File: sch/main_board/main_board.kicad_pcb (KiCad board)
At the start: 2 copper layers, 94.8 x 75.2 mm, 58 parts, among them J1 BVCC, J13 5V_GND, J14 IO23, J15 IO22, J16 IO1, J17 IO3, J18 IO21, J2 BGND, J21 5V, J22 TX2, J23 RX2, J24 12V_CUT2, J25 12V_CUT, J26 DC 12V, J27 DC 5V, J3 3.3V, J30 5V_CUT, J4 PWR_MOTOR_L, J5 PWR_MOTOR_R, J6 CUT_LOAD, J7 MOTOR_R, J8 MOTOR_L, J9 EN, Q1 BC847, Q2 K4145, Q3 K4145, Q4 BC847, Q5 K4145, Q6 BC847, Q7 K4145, Q8 BC847, Q9 K4145

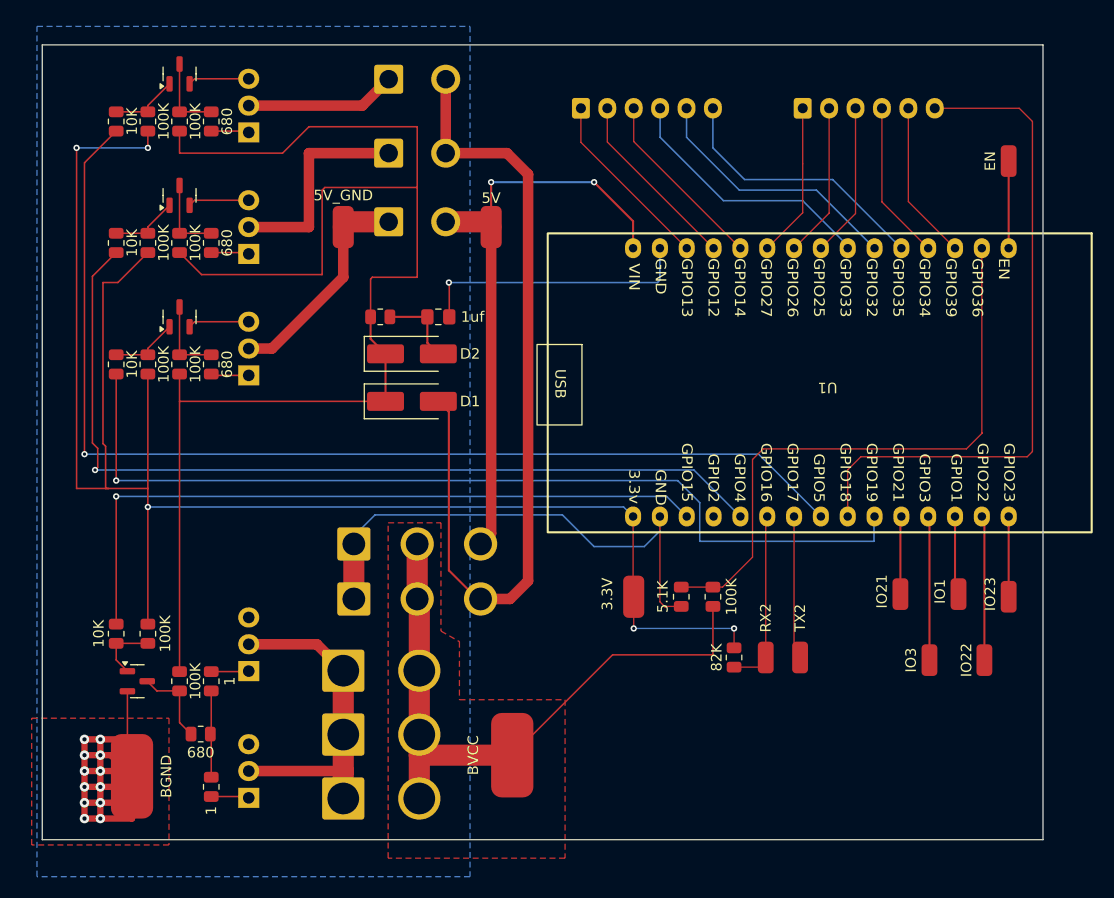
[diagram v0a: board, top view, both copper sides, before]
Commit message: Final scheme changes before production
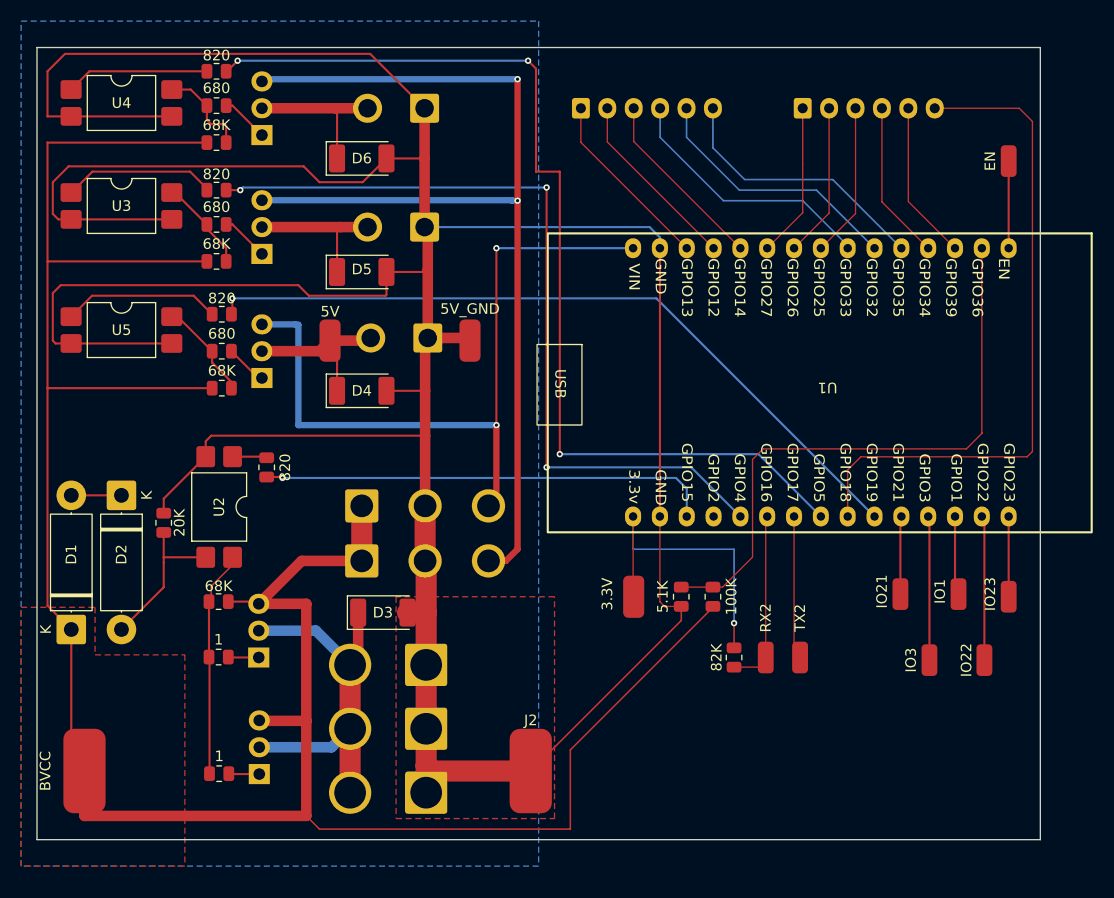
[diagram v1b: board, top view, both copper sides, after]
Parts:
- removed C1: 1uf, Capacitor_SMD:C_0805_2012Metric_Pad1.18x1.45mm_HandSolder
- removed Q6, Q8: BC847, Package_TO_SOT_SMD:SOT-23
- removed Q7, Q9: K4145, Package_TO_SOT_THT:TO-220-3_Vertical
- removed R15: 10K, Resistor_SMD:R_0805_2012Metric
- removed R16, R17: 100K, Resistor_SMD:R_0805_2012Metric
- removed R18: 680, Resistor_SMD:R_0805_2012Metric
- removed R21: 100, Resistor_SMD:R_0805_2012Metric
- added D3: D, Diode_SMD:D_2010_5025Metric_Pad1.52x2.65mm_HandSolder, F.Cu at (88.8, 93.5)
- added D4: D, Diode_SMD:D_2010_5025Metric_Pad1.52x2.65mm_HandSolder, F.Cu at (86.8, 72.5)
- added D5: D, Diode_SMD:D_2010_5025Metric_Pad1.52x2.65mm_HandSolder, F.Cu at (86.8, 61.2)
- added D6: D, Diode_SMD:D_2010_5025Metric_Pad1.52x2.65mm_HandSolder, F.Cu at (86.8, 50.5)
- added U2: EL817, Package_DIP:SMDIP-4_W9.53mm, F.Cu at (73.2, 83.5)
- added U3: EL817, Package_DIP:SMDIP-4_W9.53mm, F.Cu at (64.0, 55.0)
- added U4: EL817, Package_DIP:SMDIP-4_W9.53mm, F.Cu at (64.0, 45.2)
- added U5: EL817, Package_DIP:SMDIP-4_W9.53mm, F.Cu at (64.0, 66.8)
- D1, D2: value D -> 5.1; footprint Diode_SMD:D_SMA_Handsoldering -> Diode_THT:D_5W_P12.70mm_Horizontal
- Q1, Q4: value BC847 -> IRF4905; footprint Package_TO_SOT_SMD:SOT-23 -> Package_TO_SOT_THT:TO-220-3_Vertical; moved to B.Cu
- Q2, Q3, Q5: value K4145 -> IRF4905
- R1: value 10K -> 20K
- R10: value 680 -> 1
- R11: value 10K -> 1
- R12, R13: value 100K -> 680
- R2, R9: value 100K -> 68K
- R3, R8: value 100K -> 820
- R4: value 680 -> 820
- R5: value 1 -> 68K
- R6: value 1 -> 820
- R7: value 10K -> 68K
- moved R6 67.8 mm to (73.0, 42.2), turned to 0 degrees
- moved Q3 62.8 mm to (77.3, 48.3)
- moved R4 51.5 mm to (73.0, 53.5)
- moved R11 51.2 mm to (73.2, 108.8), turned to 180 degrees
- moved J1 40.5 mm to (60.5, 108.5)
- moved R5 39.8 mm to (73.0, 60.2), turned to 180 degrees
- moved Q2 39.5 mm to (77.3, 59.5)
- moved D1 38.8 mm to (59.2, 95.1), turned to 90 degrees
- moved Q5 37.8 mm to (77.0, 108.8)
- moved J2 37.8 mm to (102.8, 108.5)
- moved D2 30.6 mm to (64.0, 82.4), turned to -90 degrees
- moved R10 27.7 mm to (73.2, 97.7), turned to 180 degrees
- moved R7 23.0 mm to (73.0, 49.0), turned to 180 degrees
- moved R3 21.9 mm to (77.8, 79.8), turned to -90 degrees
- moved J21 18.7 mm to (83.8, 67.8)
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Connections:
- D1 pad 1: MF_VCC -> VCC
- D1 pad 2: +12V -> Net-(D1-A)
- D2 pad 1: MF_VCC -> Net-(D1-A)
- D2 pad 2: Net-(D2-A) -> MF_GND
- J13 pad 1: Net-(J13-Pin_1) -> GND
- J21 pad 1: +5V -> Net-(D4-K)
- J24 pad 1: Net-(J24-Pin_1) -> GND
- J24 pad 2: +12V -> Net-(D6-K)
- J25 pad 1: Net-(J25-Pin_1) -> GND
- J25 pad 2: +12V -> Net-(D5-K)
- J26 pad 1: GND -> VCC
- J26 pad 2: VCC -> GND
- J27 pad 1: GND -> VCC
- J27 pad 2: VCC -> GND
- J30 pad 1: Net-(J13-Pin_1) -> GND
- J30 pad 2: +5V -> Net-(D4-K)
- J4 pad 1: Net-(J4-Pin_1) -> GND
- J4 pad 2: VCC -> Net-(D3-K)
- J5 pad 1: Net-(J4-Pin_1) -> GND
- J5 pad 2: VCC -> Net-(D3-K)
- J6 pad 1: Net-(J4-Pin_1) -> GND
- J6 pad 2: VCC -> Net-(D3-K)
- Q1 pad 1: Net-(Q1-B) -> Net-(Q1-G)
- Q1 pad 2: GND -> Net-(D3-K)
- Q1 pad 3: Net-(Q1-C) -> VCC
- Q2 pad 2: Net-(J4-Pin_1) -> Net-(D5-K)
- Q2 pad 3: GND -> +12V
- Q3 pad 2: Net-(J4-Pin_1) -> Net-(D6-K)
- Q3 pad 3: GND -> +12V
- Q4 pad 1: Net-(Q4-B) -> Net-(Q4-G)
- Q4 pad 2: GND -> Net-(D4-K)
- Q4 pad 3: Net-(Q4-C) -> +5V
- Q5 pad 2: Net-(J13-Pin_1) -> Net-(D3-K)
- Q5 pad 3: GND -> VCC
- R1 pad 1: VCC_CUT -> GND
- R1 pad 2: Net-(Q1-B) -> MF_GND
- R10 pad 1: Net-(Q4-C) -> Net-(Q1-G)
- R10 pad 2: Net-(Q5-G) -> Net-(R10-Pad2)
- R11 pad 1: 12V_CUT -> Net-(Q5-G)
- R11 pad 2: Net-(Q6-B) -> Net-(R10-Pad2)
- R12 pad 1: Net-(Q6-B) -> Net-(Q4-G)
- R12 pad 2: +3.3V -> Net-(R12-Pad2)
- R13 pad 1: Net-(Q6-C) -> Net-(Q2-G)
- R13 pad 2: MF_VCC -> Net-(R13-Pad2)
- R14 pad 1: Net-(Q6-C) -> Net-(Q3-G)
- R14 pad 2: Net-(Q7-G) -> Net-(R14-Pad2)
- R2 pad 1: Net-(Q1-B) -> Net-(R10-Pad2)
- R2 pad 2: +3.3V -> VCC
- R3 pad 1: Net-(Q1-C) -> Net-(R3-Pad1)
- R3 pad 2: MF_VCC -> VCC_CUT
- R4 pad 1: Net-(Q1-C) -> Net-(R4-Pad1)
- R4 pad 2: Net-(R4-Pad2) -> 12V_CUT
- R5 pad 1: Net-(R4-Pad2) -> Net-(R13-Pad2)
- R5 pad 2: Net-(Q2-G) -> VCC
- R6 pad 1: Net-(R4-Pad2) -> Net-(R6-Pad1)
- R6 pad 2: Net-(Q3-G) -> 12V_CUT2
- R7 pad 1: 5V_CUT -> Net-(R14-Pad2)
- R7 pad 2: Net-(Q4-B) -> VCC
- R8 pad 1: Net-(Q4-B) -> Net-(R8-Pad1)
- R8 pad 2: +3.3V -> 5V_CUT
- R9 pad 1: Net-(Q4-C) -> Net-(R12-Pad2)
- R9 pad 2: MF_VCC -> VCC
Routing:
- net GND: track 155.7 -> 359.0 mm, vias 13 -> 0
- net VCC: track 60.5 -> 232.8 mm
- net MF_VCC: track 135.7 -> 0.00 mm
- net +3.3V: track 164.6 -> 29.6 mm, vias 5 -> 1
- net Net-(D3-K): track 0.00 -> 36.7 mm
- net Net-(J4-Pin_1): track 31.0 -> 0.00 mm
- net VCC_CUT: track 66.9 -> 42.9 mm
- net Net-(R10-Pad2): track 0.00 -> 21.4 mm
- net Net-(J13-Pin_1): track 21.0 -> 0.00 mm
- net Net-(J25-Pin_1): track 20.2 -> 0.00 mm
- net 5V_CUT: track 88.8 -> 70.9 mm
- net +12V: track 79.9 -> 96.5 mm, vias 0 -> 2
- net Net-(D4-K): track 0.00 -> 15.8 mm
- net Net-(R8-Pad1): track 0.00 -> 14.9 mm
- net MF_GND: track 0.00 -> 14.8 mm
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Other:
- board size 94.8 x 75.2 mm -> 95 x 75 mm
